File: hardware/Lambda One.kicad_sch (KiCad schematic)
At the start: 20 parts, among them IC1 01, J1 Conn_01x02, SW1 SW_Push, U1 W65C816SxP, U3 ATF22V10C, U6 74AHC1G04, Y1 TFT680

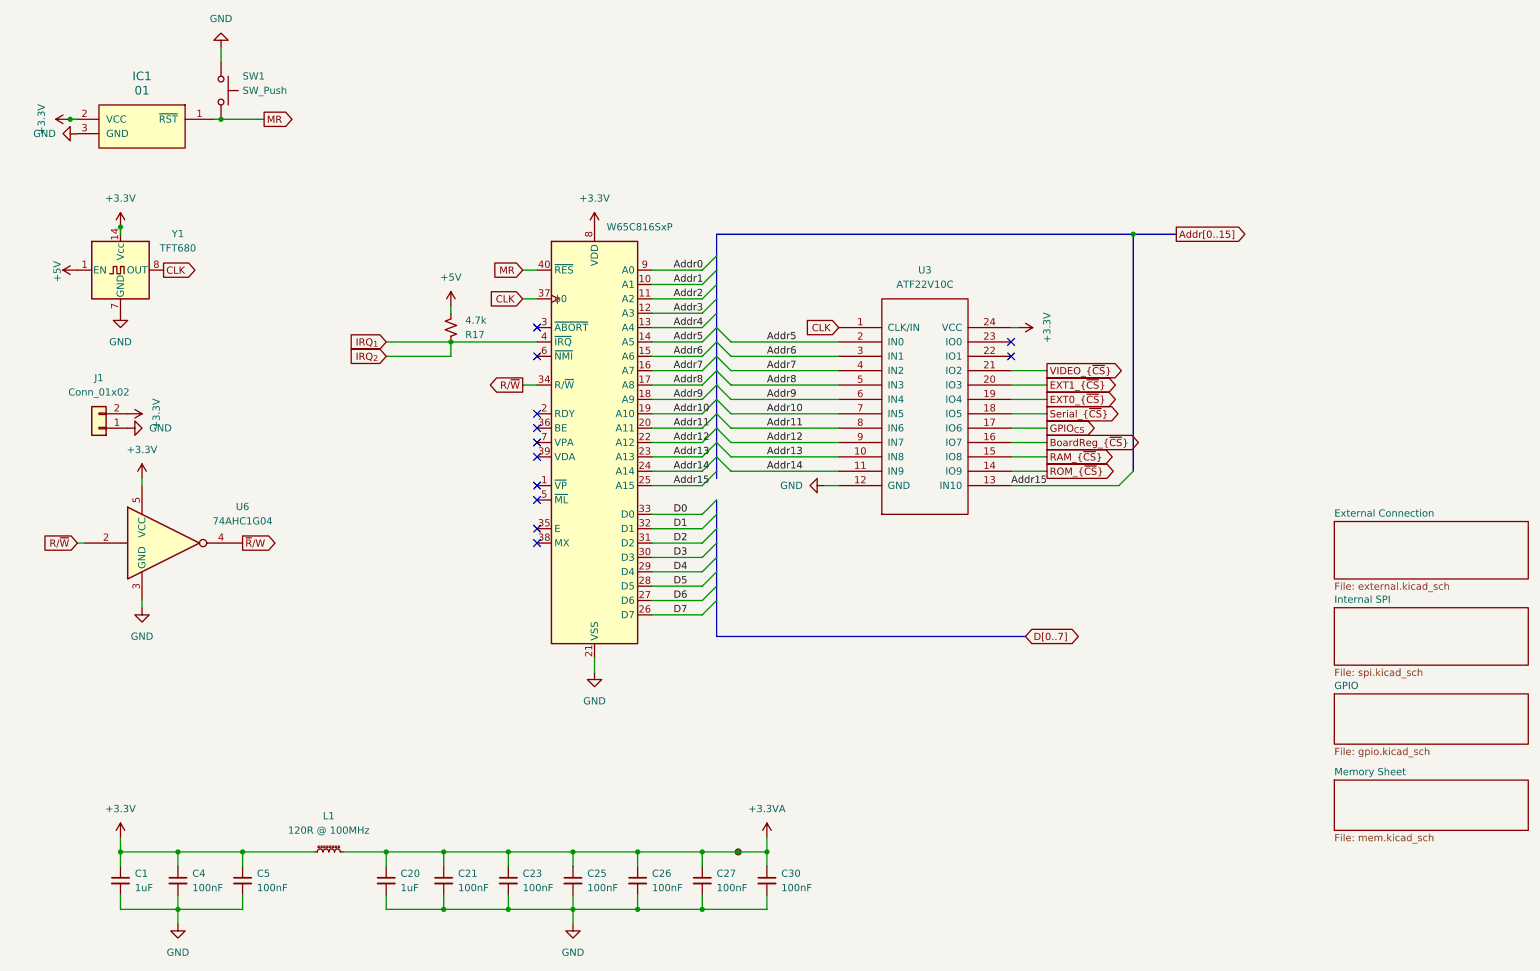
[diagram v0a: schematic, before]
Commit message: Fixed all erros and warning
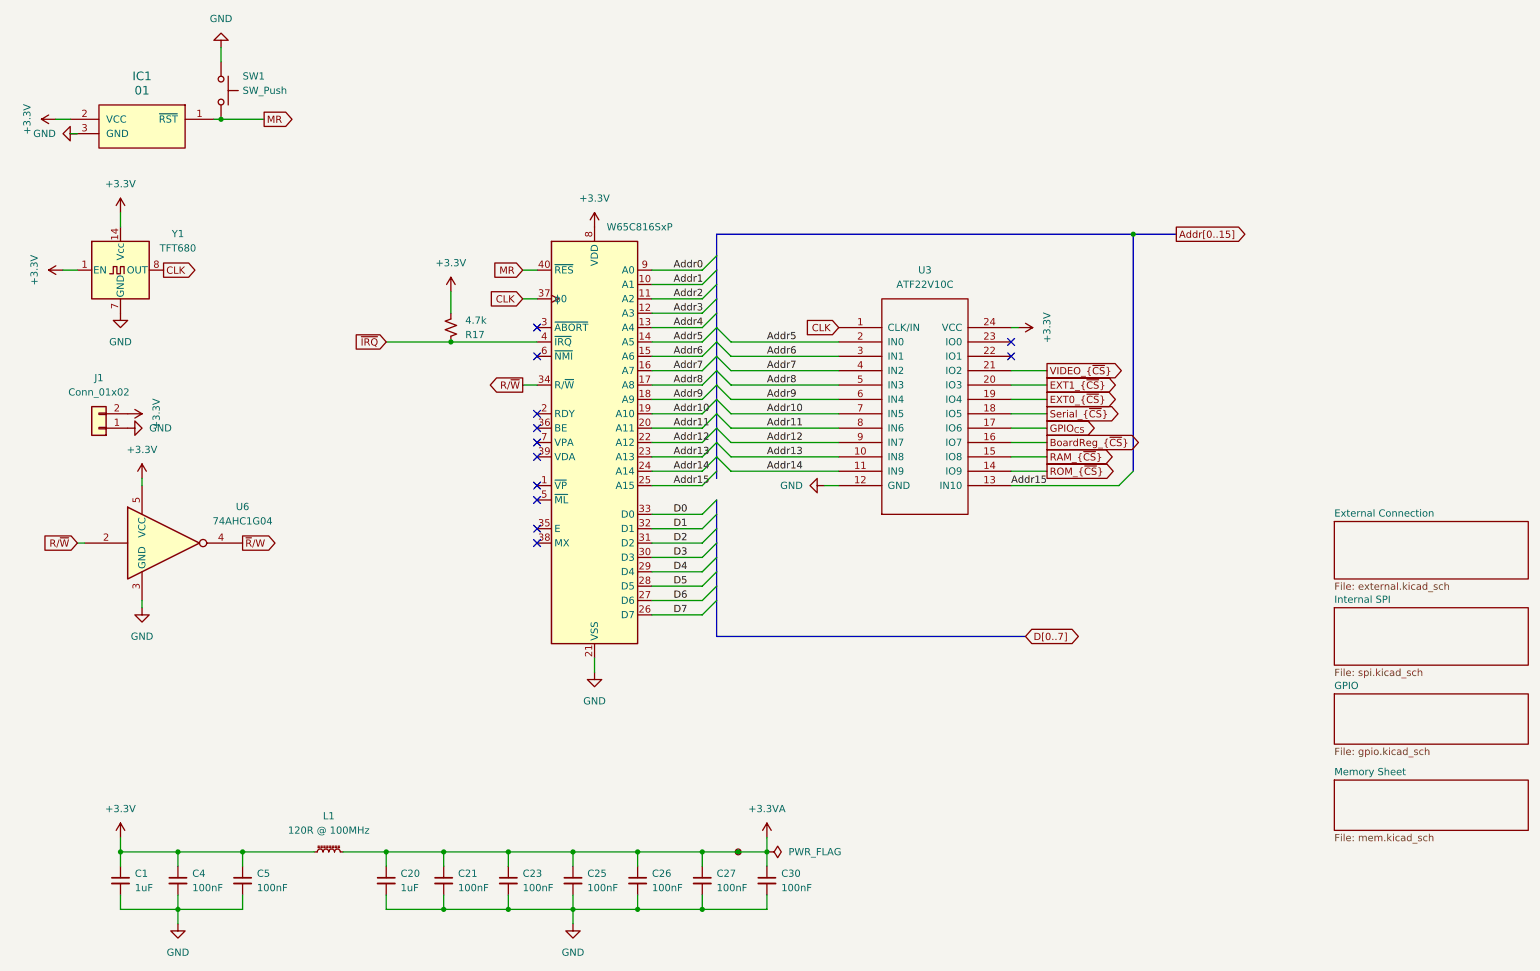
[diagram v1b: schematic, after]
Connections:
- net +5V is gone; now on net +3.3V: R17.2, Y1.1 (EN)
- net IRQ_{1} renamed ~{IRQ}
